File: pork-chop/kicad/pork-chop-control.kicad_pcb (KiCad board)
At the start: 2 copper layers, 88 x 71 mm, 35 parts, among them J1 MUSBD111M0, J2 left, J3 right, SW1 RESET, U1 ATmega32U2, U2 USBLC6-2SC6, Y1 16MHz

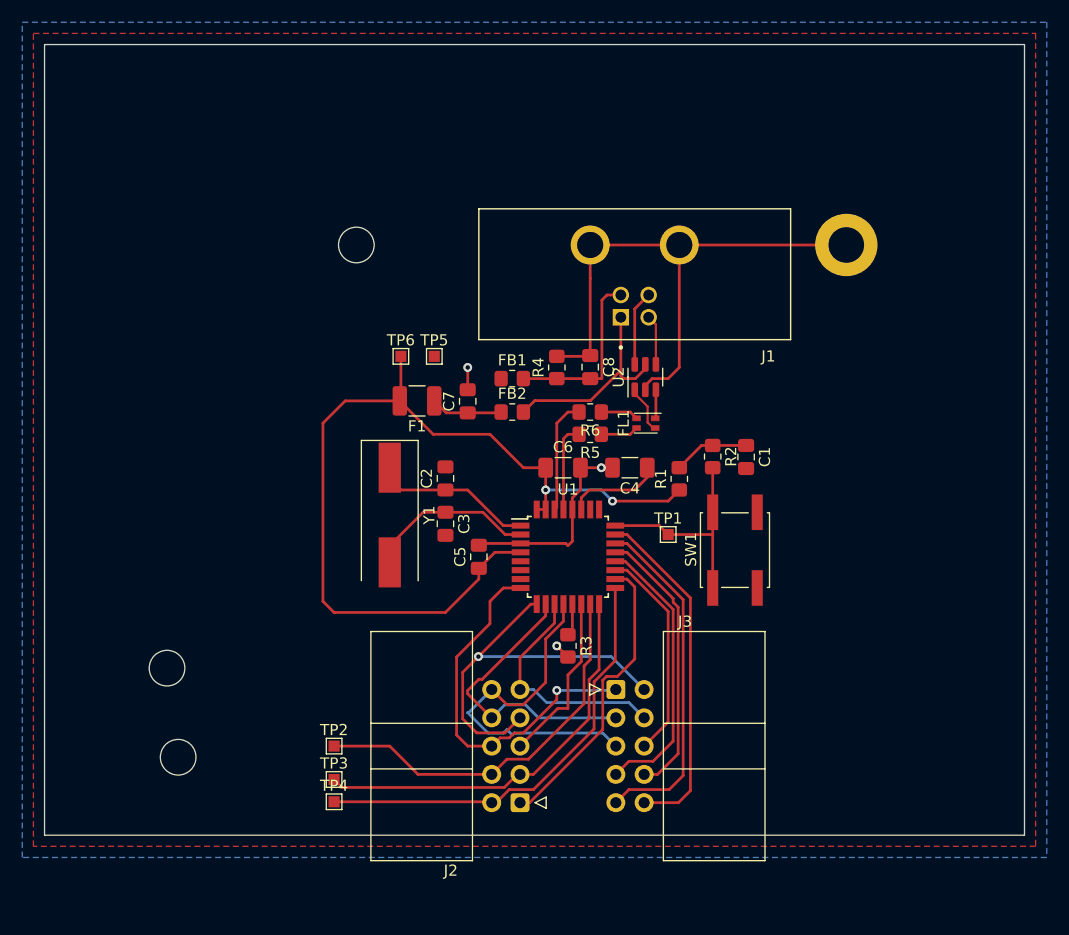
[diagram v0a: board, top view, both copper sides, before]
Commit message: routing
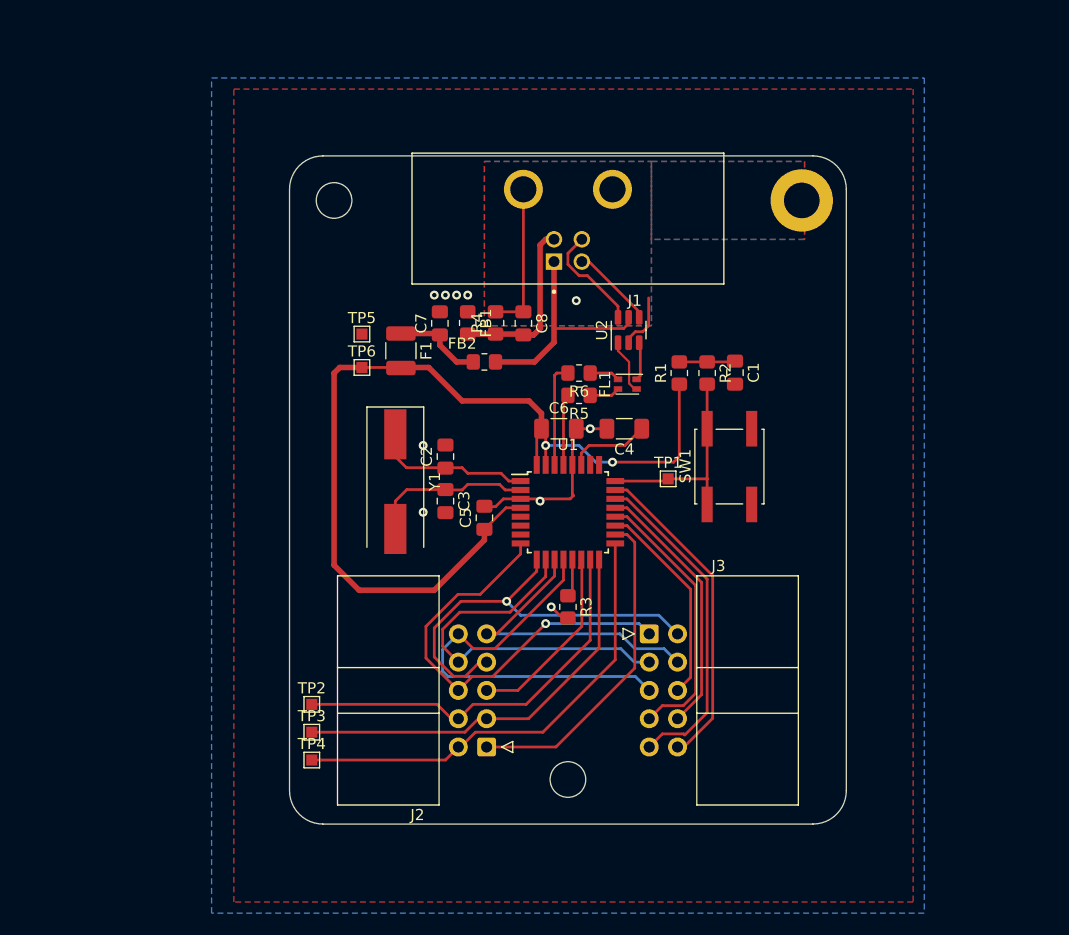
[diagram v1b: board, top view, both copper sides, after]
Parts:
- removed the REF** at (89.0, 106.0)
- moved REF** 35.1 mm to (125.0, 116.0)
- moved R1 9.50 mm to (135.0, 79.5)
- moved J1 7.81 mm to (125.0, 63.0)
- moved C1 7.64 mm to (140.0, 79.5)
- moved R2 7.52 mm to (137.5, 79.5)
- moved SW1 7.52 mm to (139.5, 87.9)
- moved C7 7.43 mm to (113.5, 75.0)
- moved C8 7.17 mm to (121.0, 75.0)
- moved R4 6.80 mm to (118.5, 75.0)
- moved TP5 6.80 mm to (106.5, 76.0)
- moved FB1 6.40 mm to (116.0, 75.0), turned to -90 degrees
- moved J2 5.83 mm to (117.7, 113.1)
- moved J3 5.83 mm to (132.3, 102.9)
- moved H1 5.66 mm to (146.0, 64.0)
- moved FB2 5.15 mm to (117.5, 78.5)
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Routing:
- net GNDPWR: track 51.1 -> 20.1 mm, vias 0 -> 1
- net R2: track 26.3 -> 34.4 mm
- net R3: track 21.2 -> 27.9 mm
- net R4: track 31.9 -> 37.6 mm
- net R0: track 33.8 -> 39.1 mm
- net +5V: track 81.7 -> 86.7 mm
- net Net-(J1-Pad3): track 6.75 -> 9.83 mm
- net /D-: track 4.50 -> 7.52 mm
- net C0: track 26.8 -> 29.6 mm
- net GND: track 21.9 -> 19.3 mm, vias 3 -> 9
- net C4: track 15.6 -> 17.8 mm
- net C9: track 31.0 -> 29.0 mm
- net C1: track 39.6 -> 41.4 mm
- net Net-(FB2-Pad2): track 18.6 -> 20.4 mm
- net Net-(C1-Pad1): track 6.83 -> 5.03 mm
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- added copper zone on B.Cu, net GNDPWR
- added copper zone on F.Cu, net GNDPWR
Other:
- board size 88 x 71 mm -> 50 x 60 mm
